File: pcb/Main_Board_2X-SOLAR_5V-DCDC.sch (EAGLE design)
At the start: 71 parts, among them CN5 USBA_FEMALE, M3AB FDMC8030, T2 MMUN2133LT1G, U1 LTC4015EUHFPBFQFN-38_UHF-M, U3 TPS61090RSAR, X1 6V_PV

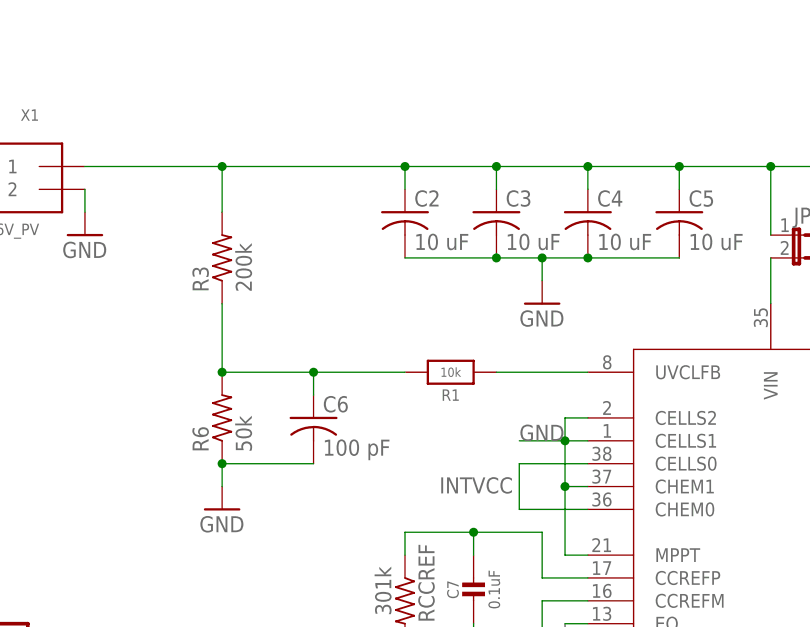
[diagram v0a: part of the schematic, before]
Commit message: OSH print V1 P2
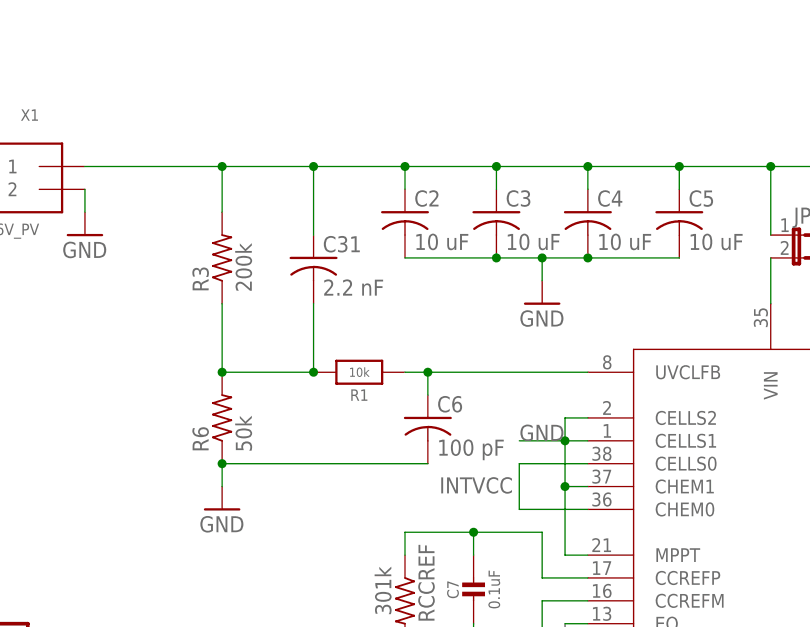
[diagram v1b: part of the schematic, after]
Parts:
- added C31: 2.2 nF, adafruit:C-USC0805
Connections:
- net N$5: now also C6.1
- net UVCLFB: now also C31.2; no longer C6.1
- net VIN: now also C31.1
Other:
- moved on the sheet: C6, R1
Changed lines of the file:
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@@
 <part name="INFET-Q1" library="TRANS_SI7635DP-T1-GE3" deviceset="SI4840DY" device=""/>
 <part name="JP2" library="jumper" library_urn="urn:adsk.eagle:library:252" deviceset="JP1E" device="" package3d_urn="urn:adsk.eagle:package:15455/1"/>
+<part name="C31" library="adafruit" library_urn="urn:adsk.eagle:library:420" deviceset="C-US" device="C0805" value="2.2 nF"/>
 </parts>
 <sheets>
@@
 <instance part="C4" gate="G$1" x="76.2" y="147.32"/>
 <instance part="C5" gate="G$1" x="86.36" y="147.32"/>
-<instance part="C6" gate="G$1" x="45.72" y="124.46"/>
+<instance part="C6" gate="G$1" x="58.42" y="124.46"/>
 <instance part="R6" gate="G$1" x="35.56" y="124.46" rot="R90"/>
 <instance part="GND3" gate="1" x="35.56" y="114.3"/>
@@
 <instance part="CN1" gate="G$1" x="236.22" y="45.72"/>
 <instance part="U$12" gate="G$1" x="226.06" y="40.64"/>
-<instance part="R1" gate="G$1" x="60.96" y="129.54" rot="R180"/>
+<instance part="R1" gate="G$1" x="50.8" y="129.54" rot="R180"/>
 <instance part="C29" gate="G$1" x="236.22" y="147.32" smashed="yes">
 <attribute name="NAME" x="238.76" y="150.876" size="1.27" layer="95" font="vector"/>
@@
 <instance part="INFET-Q1" gate="G$1" x="124.46" y="152.4" rot="MR90"/>
 <instance part="JP2" gate="A" x="99.06" y="144.78" rot="R270"/>
+<instance part="C31" gate="G$1" x="45.72" y="142.24"/>
 </instances>
 <busses>
@@
 <pinref part="GND3" gate="1" pin="GND"/>
 <pinref part="C6" gate="G$1" pin="2"/>
-<wire x1="45.72" y1="119.38" x2="35.56" y2="119.38" width="0.1524" layer="91"/>
+<wire x1="58.42" y1="119.38" x2="35.56" y2="119.38" width="0.1524" layer="91"/>
 <junction x="35.56" y="119.38"/>
 <wire x1="35.56" y1="119.38" x2="35.56" y2="116.84" width="0.1524" layer="91"/>
@@
 <net name="UVCLFB" class="0">
 <segment>
-<pinref part="C6" gate="G$1" pin="1"/>
-<wire x1="45.72" y1="129.54" x2="45.72" y2="127" width="0.1524" layer="91"/>
 <pinref part="R6" gate="G$1" pin="2"/>
 <wire x1="45.72" y1="129.54" x2="35.56" y2="129.54" width="0.1524" layer="91"/>
@@
 <wire x1="35.56" y1="129.54" x2="35.56" y2="137.16" width="0.1524" layer="91"/>
 <pinref part="R1" gate="G$1" pin="2"/>
-<wire x1="45.72" y1="129.54" x2="55.88" y2="129.54" width="0.1524" layer="91"/>
+<pinref part="C31" gate="G$1" pin="2"/>
+<wire x1="45.72" y1="137.16" x2="45.72" y2="129.54" width="0.1524" layer="91"/>
 <junction x="45.72" y="129.54"/>
 </segment>
@@
 <junction x="55.88" y="152.4"/>
 <pinref part="R3" gate="G$1" pin="2"/>
-<wire x1="35.56" y1="152.4" x2="55.88" y2="152.4" width="0.1524" layer="91"/>
+<wire x1="35.56" y1="152.4" x2="45.72" y2="152.4" width="0.1524" layer="91"/>
+<wire x1="45.72" y1="152.4" x2="55.88" y2="152.4" width="0.1524" layer="91"/>
 <wire x1="35.56" y1="147.32" x2="35.56" y2="152.4" width="0.1524" layer="91"/>
 <junction x="35.56" y="152.4"/>
 <pinref part="INFET-Q1" gate="G$1" pin="S"/>
 <pinref part="JP2" gate="A" pin="1"/>
+<pinref part="C31" gate="G$1" pin="1"/>
+<wire x1="45.72" y1="144.78" x2="45.72" y2="152.4" width="0.1524" layer="91"/>
+<junction x="45.72" y="152.4"/>
 </segment>
 </net>
@@
 <pinref part="R1" gate="G$1" pin="1"/>
 <pinref part="U1" gate="A" pin="UVCLFB"/>
-<wire x1="66.04" y1="129.54" x2="76.2" y2="129.54" width="0.1524" layer="91"/>
-</segment>
-</net>
+<wire x1="55.88" y1="129.54" x2="58.42" y2="129.54" width="0.1524" layer="91"/>
+<pinref part="C6" gate="G$1" pin="1"/>
+<wire x1="58.42" y1="129.54" x2="76.2" y2="129.54" width="0.1524" layer="91"/>
+<wire x1="58.42" y1="127" x2="58.42" y2="129.54" width="0.1524" layer="91"/>
+<junction x="58.42" y="129.54"/>
+</segment>
+</net>
